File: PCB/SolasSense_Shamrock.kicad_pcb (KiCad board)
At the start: 2 copper layers, 86.7 x 75 mm, 15 parts, among them U1 ESP32-C3_SUPERMINI_TH

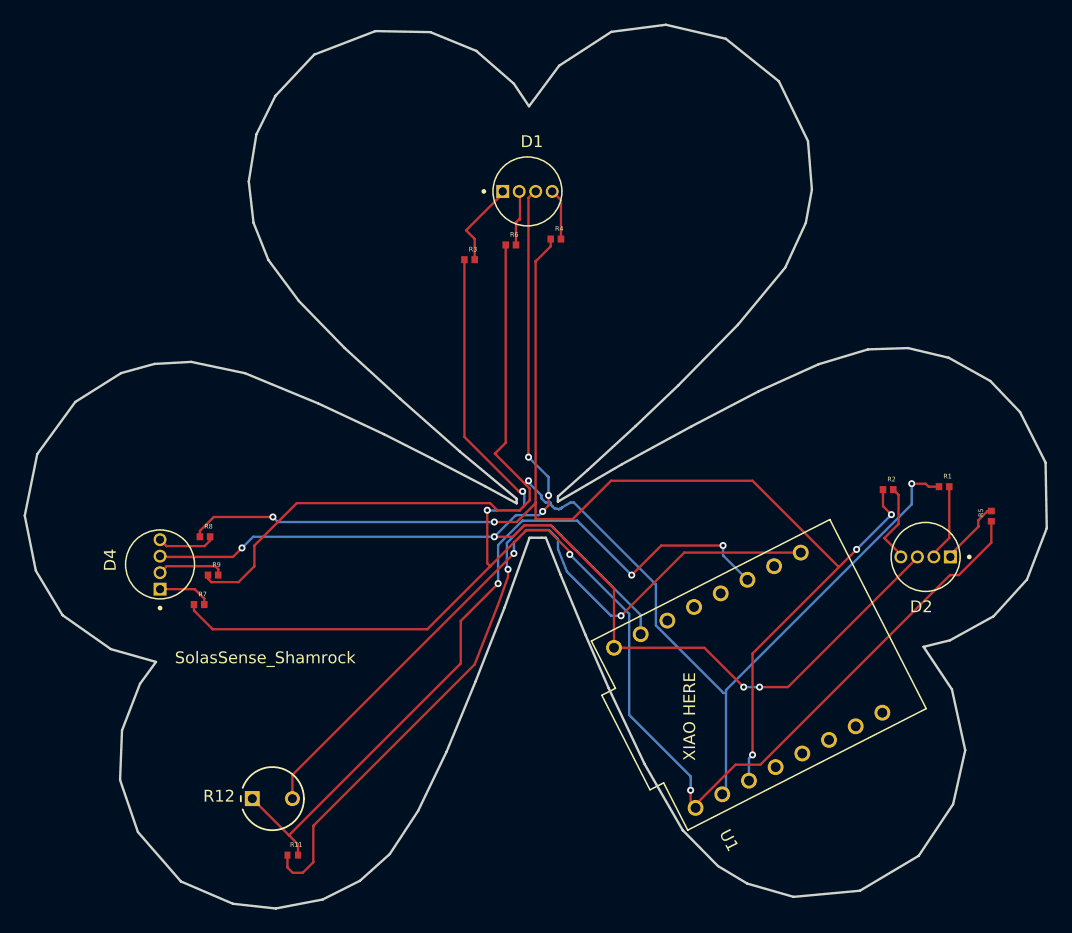
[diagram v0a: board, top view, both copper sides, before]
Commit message: Add files via upload
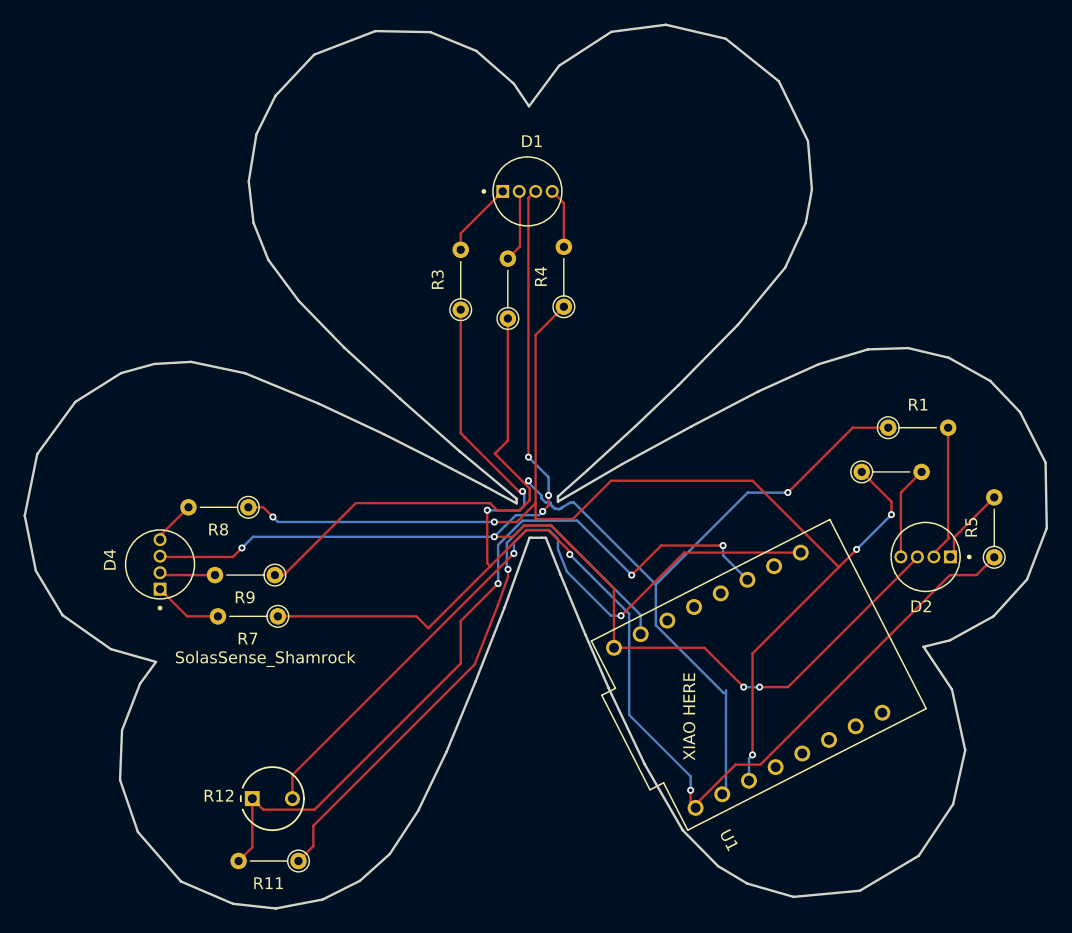
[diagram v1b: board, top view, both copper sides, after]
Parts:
- R1, R2, R3, R4, R5, R6, R7, R8, R9: footprint Resistor 220:RESC1005X35N -> Resistor_THT:R_Axial_DIN0204_L3.6mm_D1.6mm_P5.08mm_Vertical
- R11: footprint Resistor 10k:RESC1005X40N -> Resistor_THT:R_Axial_DIN0204_L3.6mm_D1.6mm_P5.08mm_Vertical
- moved R1 6.89 mm to (183.5, 80.0)
- moved R7 6.75 mm to (131.7, 96.0), turned to 180 degrees
- moved R6 6.25 mm to (151.2, 70.7), turned to 90 degrees
- moved R4 5.78 mm to (156.0, 69.7), turned to 90 degrees
- moved R9 5.24 mm to (131.5, 92.5), turned to 180 degrees
- moved R8 4.44 mm to (129.2, 86.8), turned to 180 degrees
- moved R3 4.31 mm to (147.2, 70.0), turned to 90 degrees
- moved R5 3.50 mm to (192.5, 91.0)
- moved R2 2.70 mm to (181.3, 83.8)
- moved R11 0.70 mm to (133.5, 116.8), turned to 180 degrees
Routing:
- net Net-(U1-GPIO6): track 118.2 -> 103.4 mm
- net Net-(U1-GPIO5): track 131.1 -> 117.1 mm
- net Net-(U1-GPIO7): track 114.8 -> 107.0 mm
- net Net-(D2-Pad2): track 6.69 -> 11.7 mm
- net GND: track 53.9 -> 50.5 mm
- net Net-(U1-GPIO2): track 65.0 -> 67.0 mm
- net Net-(D1-Pad2): track 4.82 -> 6.12 mm
- net Net-(D4-Pad1): track 4.58 -> 5.86 mm
- net Net-(D4-Pad4): track 4.99 -> 3.74 mm
- net Net-(D1-Pad1): track 7.46 -> 6.42 mm
- net Net-(D4-Pad2): track 5.77 -> 4.74 mm
- net Net-(D2-Pad1): track 5.64 -> 6.59 mm
- net Net-(D2-Pad4): track 7.05 -> 7.94 mm
- net Net-(D1-Pad4): track 4.35 -> 5.11 mm
